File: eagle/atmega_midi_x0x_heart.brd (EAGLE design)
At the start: 100 x 80 mm, 40 parts, among them J11_VCF_CUTOFF 22-23-2021, U1 ATMEGA328P_PDIP, U2 TLV2372IP

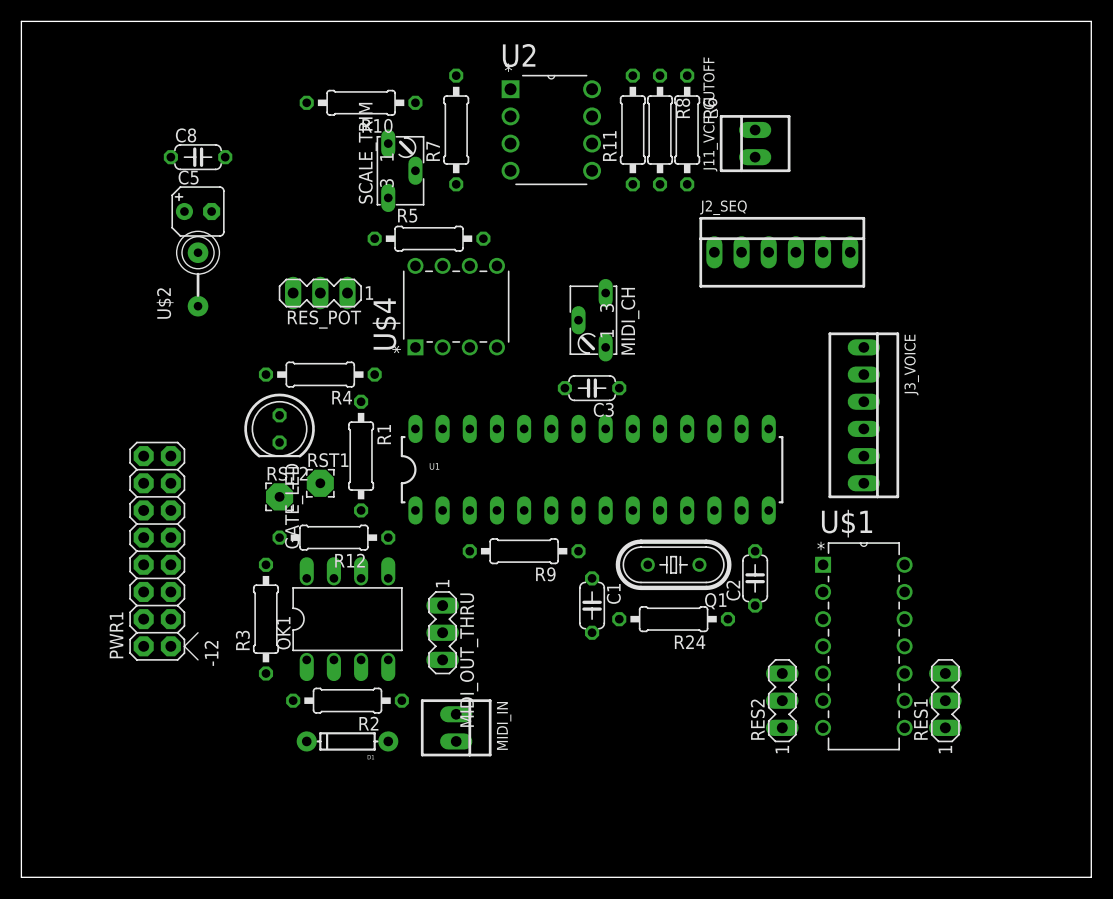
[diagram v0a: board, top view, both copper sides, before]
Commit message: almost
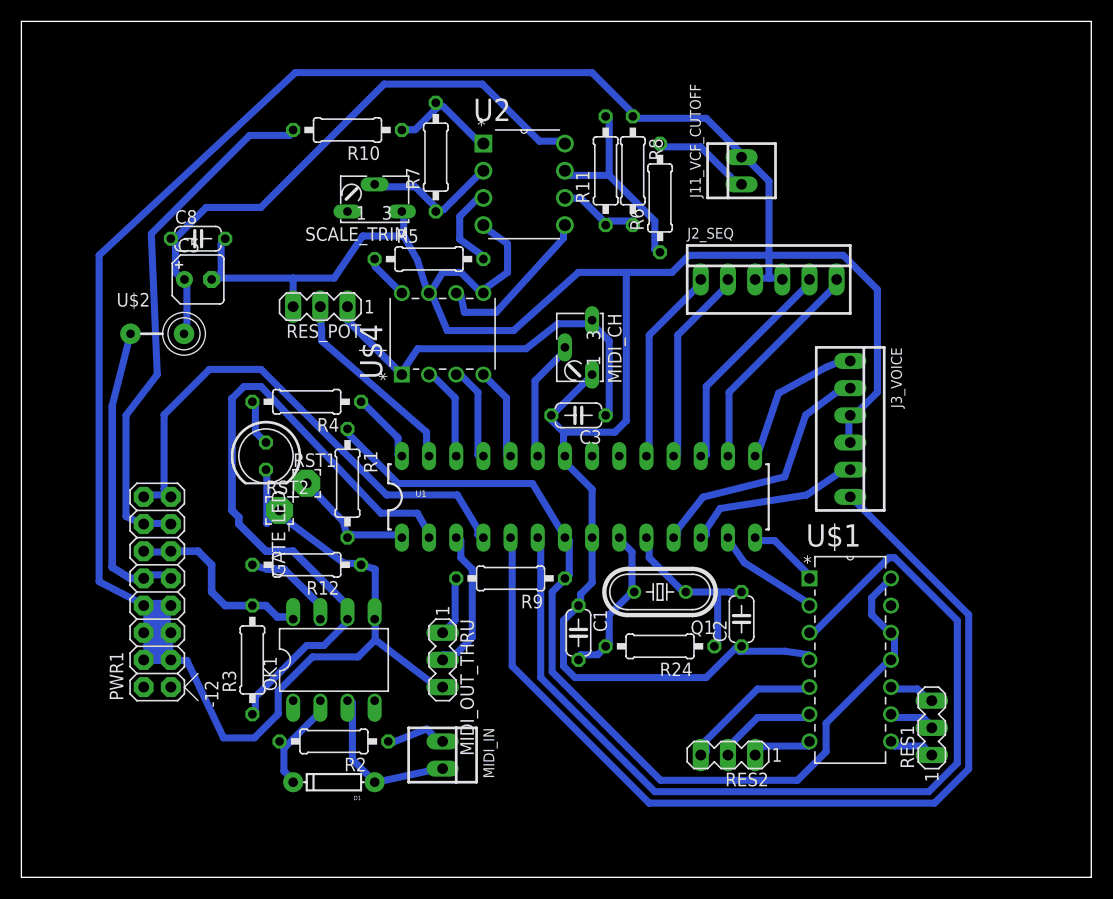
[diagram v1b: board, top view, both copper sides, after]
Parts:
- moved C8 7.62 mm to (16.5, 59.7)
- moved RES2 7.18 mm to (66.0, 11.4), turned to 180 degrees
- moved R6 6.84 mm to (59.7, 63.5), turned to 90 degrees
- moved U$2 6.35 mm to (12.7, 50.8), turned to 0 degrees
- moved C5 6.35 mm to (16.5, 55.9)
- moved U2 5.68 mm to (50.8, 61.0)
- moved R11 4.58 mm to (54.6, 66.0)
- moved R8 4.58 mm to (57.1, 66.0)
- moved SCALE_TRIM 4.02 mm to (33.0, 62.2), turned to 180 degrees
- moved R2 4.02 mm to (29.2, 12.7)
- moved C2 4.02 mm to (67.3, 24.1)
- moved D1 4.02 mm to (29.2, 8.89)
- moved OK1 4.02 mm to (29.2, 20.3)
- moved R3 4.02 mm to (21.6, 20.3)
- moved PWR1 3.81 mm to (12.7, 24.1)
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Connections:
- new net N$46: U1.21
- net +5V: no longer U1.21
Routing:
- net GND: track 0.00 -> 388.1 mm
- net +5V: track 0.00 -> 147.3 mm
- net N$1: track 0.00 -> 91.4 mm
- net N$22: track 0.00 -> 90.1 mm
- net N$30: track 0.00 -> 65.7 mm
- net +12V: track 0.00 -> 54.8 mm
- net N$40: track 0.00 -> 49.3 mm
- net N$15: track 0.00 -> 49.1 mm
- net N$11: track 0.00 -> 28.7 mm
- net N$10: track 0.00 -> 24.5 mm
- net N$21: track 0.00 -> 20.9 mm
- net N$23: track 0.00 -> 20.8 mm
- net N$17: track 0.00 -> 19.3 mm
- net N$20: track 0.00 -> 18.8 mm
- net N$38: track 0.00 -> 18.7 mm
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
